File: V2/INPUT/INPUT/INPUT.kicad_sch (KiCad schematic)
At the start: 45 parts, among them J1 Conn_01x03, J2 USB_C_Receptacle_USB2.0_16P, J3 Conn_01x03, J4 Conn_01x03, J5 Conn_01x03, J6 Conn_01x03, J7 Conn_01x03, J8 Conn_01x03, J9 Conn_01x03, Q1 QM6006D, Q2 QM6006D, Q3 QM6006D, Q4 QM6006D, Q5 QM6006D, Q6 QM6006D, Q7 QM6006D, Q8 QM6006D, SW1 SW_SPST, SW2 SW_SPST, SW3 SW_SPST, SW4 SW_SPST, SW5 SW_SPST, SW6 SW_SPST, SW7 SW_SPST, SW8 SW_SPST, U1 USBLC6-2P6

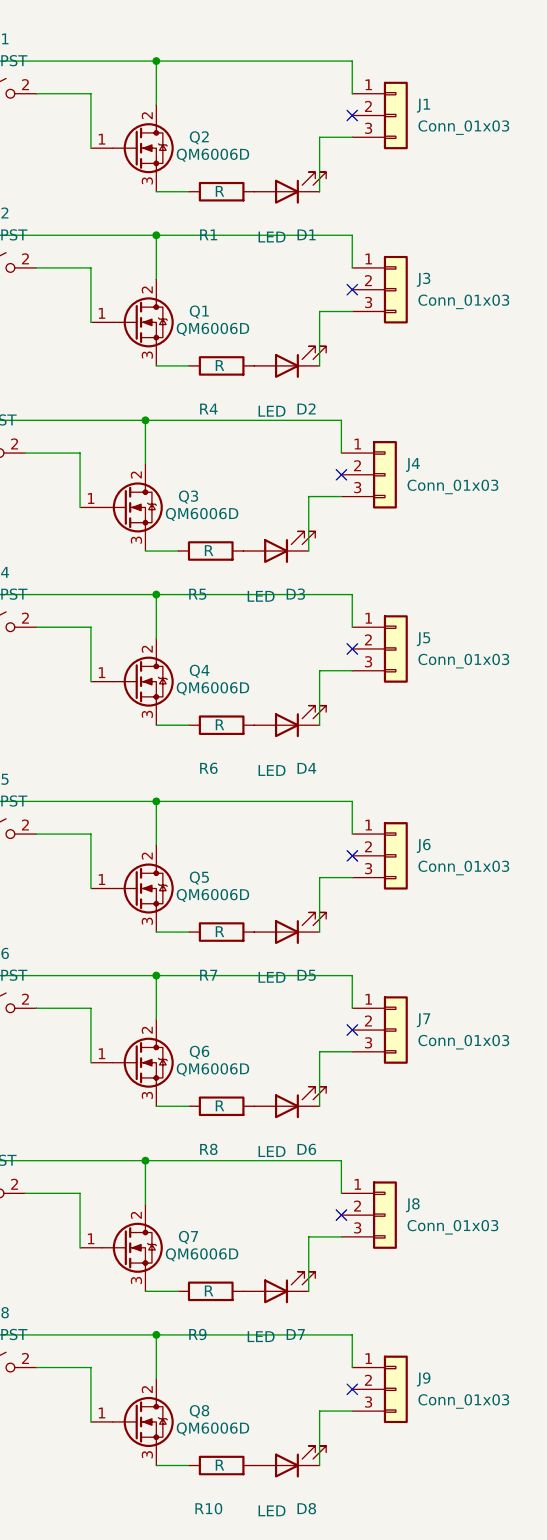
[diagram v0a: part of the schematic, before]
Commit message: Auto-update: 17.02.2026  0:08:41,99
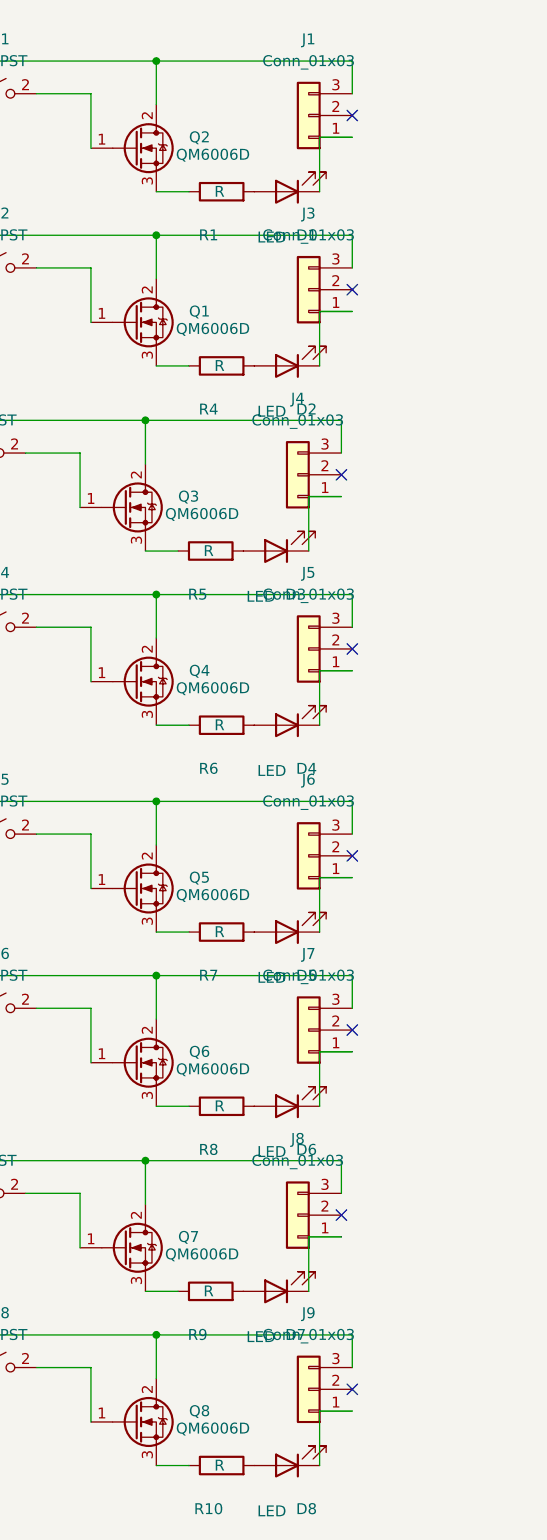
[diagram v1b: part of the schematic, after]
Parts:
- J1, J3, J4, J5, J6, J7, J8, J9: footprint Connector_JST:JST_PH_S3B-PH-K_1x03_P2.00mm_Horizontal -> Connector_PinSocket_2.54mm:PinSocket_1x03_P2.54mm_Horizontal
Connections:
- net +5V: now also J1.3 (Pin_3), J3.3 (Pin_3), J4.3 (Pin_3), J5.3 (Pin_3), J6.3 (Pin_3), J7.3 (Pin_3), J8.3 (Pin_3), J9.3 (Pin_3); no longer J1.1 (Pin_1), J3.1 (Pin_1), J4.1 (Pin_1), J5.1 (Pin_1), J6.1 (Pin_1), J7.1 (Pin_1), J8.1 (Pin_1), J9.1 (Pin_1)
- net at D6.1 (K): now also J7.1 (Pin_1); no longer J7.3 (Pin_3)
- net at D4.1 (K): now also J5.1 (Pin_1); no longer J5.3 (Pin_3)
- net at D1.1 (K): now also J1.1 (Pin_1); no longer J1.3 (Pin_3)
- net at D3.1 (K): now also J4.1 (Pin_1); no longer J4.3 (Pin_3)
- net at D2.1 (K): now also J3.1 (Pin_1); no longer J3.3 (Pin_3)
- net at D8.1 (K): now also J9.1 (Pin_1); no longer J9.3 (Pin_3)
- net at D5.1 (K): now also J6.1 (Pin_1); no longer J6.3 (Pin_3)
- net at D7.1 (K): now also J8.1 (Pin_1); no longer J8.3 (Pin_3)
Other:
- moved on the sheet: J1, J3, J4, J5, J6, J7, J8, J9

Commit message: Auto-update: 24.02.2026 16:00:58,58
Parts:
- Q1, Q2, Q3, Q4, Q5, Q6, Q7, Q8: footprint Package_TO_SOT_SMD:TO-252-2 -> Package_TO_SOT_SMD:SOT-23
- R1, R10, R2, R3, R4, R5, R6, R7, R8, R9: footprint Resistor_SMD:R_1206_3216Metric -> Resistor_SMD:R_0201_0603Metric
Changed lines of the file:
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@@
 			)
 		)
-		(property "Footprint" "Resistor_SMD:R_1206_3216Metric"
+		(property "Footprint" "Resistor_SMD:R_0201_0603Metric"
 			(at 132.08 185.928 90)
 			(effects
@@
 			)
 		)
-		(property "Footprint" "Resistor_SMD:R_1206_3216Metric"
+		(property "Footprint" "Resistor_SMD:R_0201_0603Metric"
 			(at 48.26 29.21 0)
 			(effects
@@
 			)
 		)
-		(property "Footprint" "Package_TO_SOT_SMD:TO-252-2"
+		(property "Footprint" "Package_TO_SOT_SMD:SOT-23"
 			(at 127 180.975 0)
 			(effects
@@
 			)
 		)
-		(property "Footprint" "Resistor_SMD:R_1206_3216Metric"
+		(property "Footprint" "Resistor_SMD:R_0201_0603Metric"
 			(at 132.08 144.018 90)
 			(effects
@@
 			)
 		)
-		(property "Footprint" "Resistor_SMD:R_1206_3216Metric"
+		(property "Footprint" "Resistor_SMD:R_0201_0603Metric"
 			(at 130.81 79.248 90)
 			(effects
@@
 			)
 		)
-		(property "Footprint" "Package_TO_SOT_SMD:TO-252-2"
+		(property "Footprint" "Package_TO_SOT_SMD:SOT-23"
 			(at 125.73 160.655 0)
 			(effects
@@
 			)
 		)
-		(property "Footprint" "Package_TO_SOT_SMD:TO-252-2"
+		(property "Footprint" "Package_TO_SOT_SMD:SOT-23"
 			(at 127 139.065 0)
 			(effects
@@
 			)
 		)
-		(property "Footprint" "Package_TO_SOT_SMD:TO-252-2"
+		(property "Footprint" "Package_TO_SOT_SMD:SOT-23"
 			(at 127 52.705 0)
 			(effects
@@
 			)
 		)
-		(property "Footprint" "Package_TO_SOT_SMD:TO-252-2"
+		(property "Footprint" "Package_TO_SOT_SMD:SOT-23"
 			(at 125.73 74.295 0)
 			(effects
@@
 			)
 		)
-		(property "Footprint" "Resistor_SMD:R_1206_3216Metric"
+		(property "Footprint" "Resistor_SMD:R_0201_0603Metric"
 			(at 130.81 165.608 90)
 			(effects
@@
 			)
 		)
-		(property "Footprint" "Resistor_SMD:R_1206_3216Metric"
+		(property "Footprint" "Resistor_SMD:R_0201_0603Metric"
 			(at 132.08 57.658 90)
 			(effects
@@
 			)
 		)
-		(property "Footprint" "Package_TO_SOT_SMD:TO-252-2"
+		(property "Footprint" "Package_TO_SOT_SMD:SOT-23"
 			(at 127 94.615 0)
 			(effects
@@
 			)
 		)
-		(property "Footprint" "Package_TO_SOT_SMD:TO-252-2"
+		(property "Footprint" "Package_TO_SOT_SMD:SOT-23"
 			(at 127 32.385 0)
 			(effects
@@
 			)
 		)
-		(property "Footprint" "Resistor_SMD:R_1206_3216Metric"
+		(property "Footprint" "Resistor_SMD:R_0201_0603Metric"
 			(at 132.08 123.698 90)
 			(effects
@@
 			)
 		)
-		(property "Footprint" "Resistor_SMD:R_1206_3216Metric"
+		(property "Footprint" "Resistor_SMD:R_0201_0603Metric"
 			(at 132.08 37.338 90)
 			(effects
@@
 			)
 		)
-		(property "Footprint" "Resistor_SMD:R_1206_3216Metric"
+		(property "Footprint" "Resistor_SMD:R_0201_0603Metric"
 			(at 132.08 99.568 90)
 			(effects
@@
 			)
 		)
-		(property "Footprint" "Package_TO_SOT_SMD:TO-252-2"
+		(property "Footprint" "Package_TO_SOT_SMD:SOT-23"
 			(at 127 118.745 0)
 			(effects
@@
 			)
 		)
-		(property "Footprint" "Resistor_SMD:R_1206_3216Metric"
+		(property "Footprint" "Resistor_SMD:R_0201_0603Metric"
 			(at 48.26 31.75 0)
 			(effects

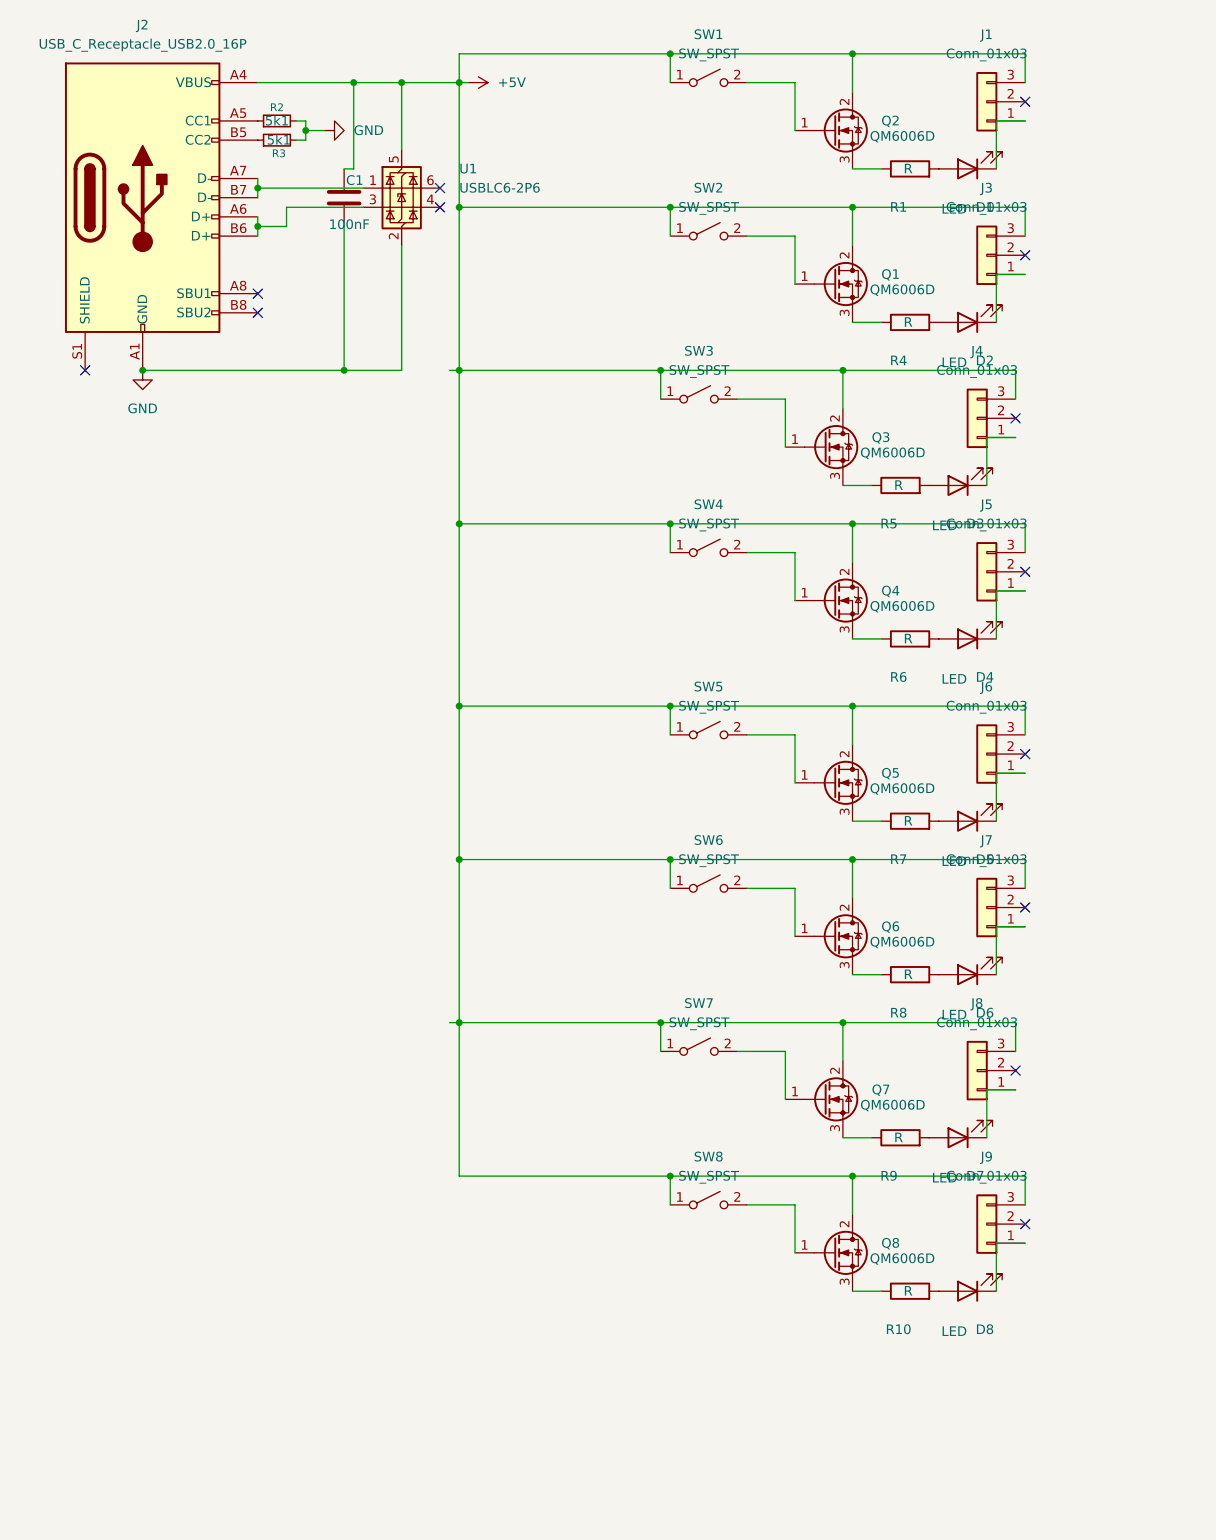
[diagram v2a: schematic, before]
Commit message: Auto-update: 26.02.2026  0:22:57,46
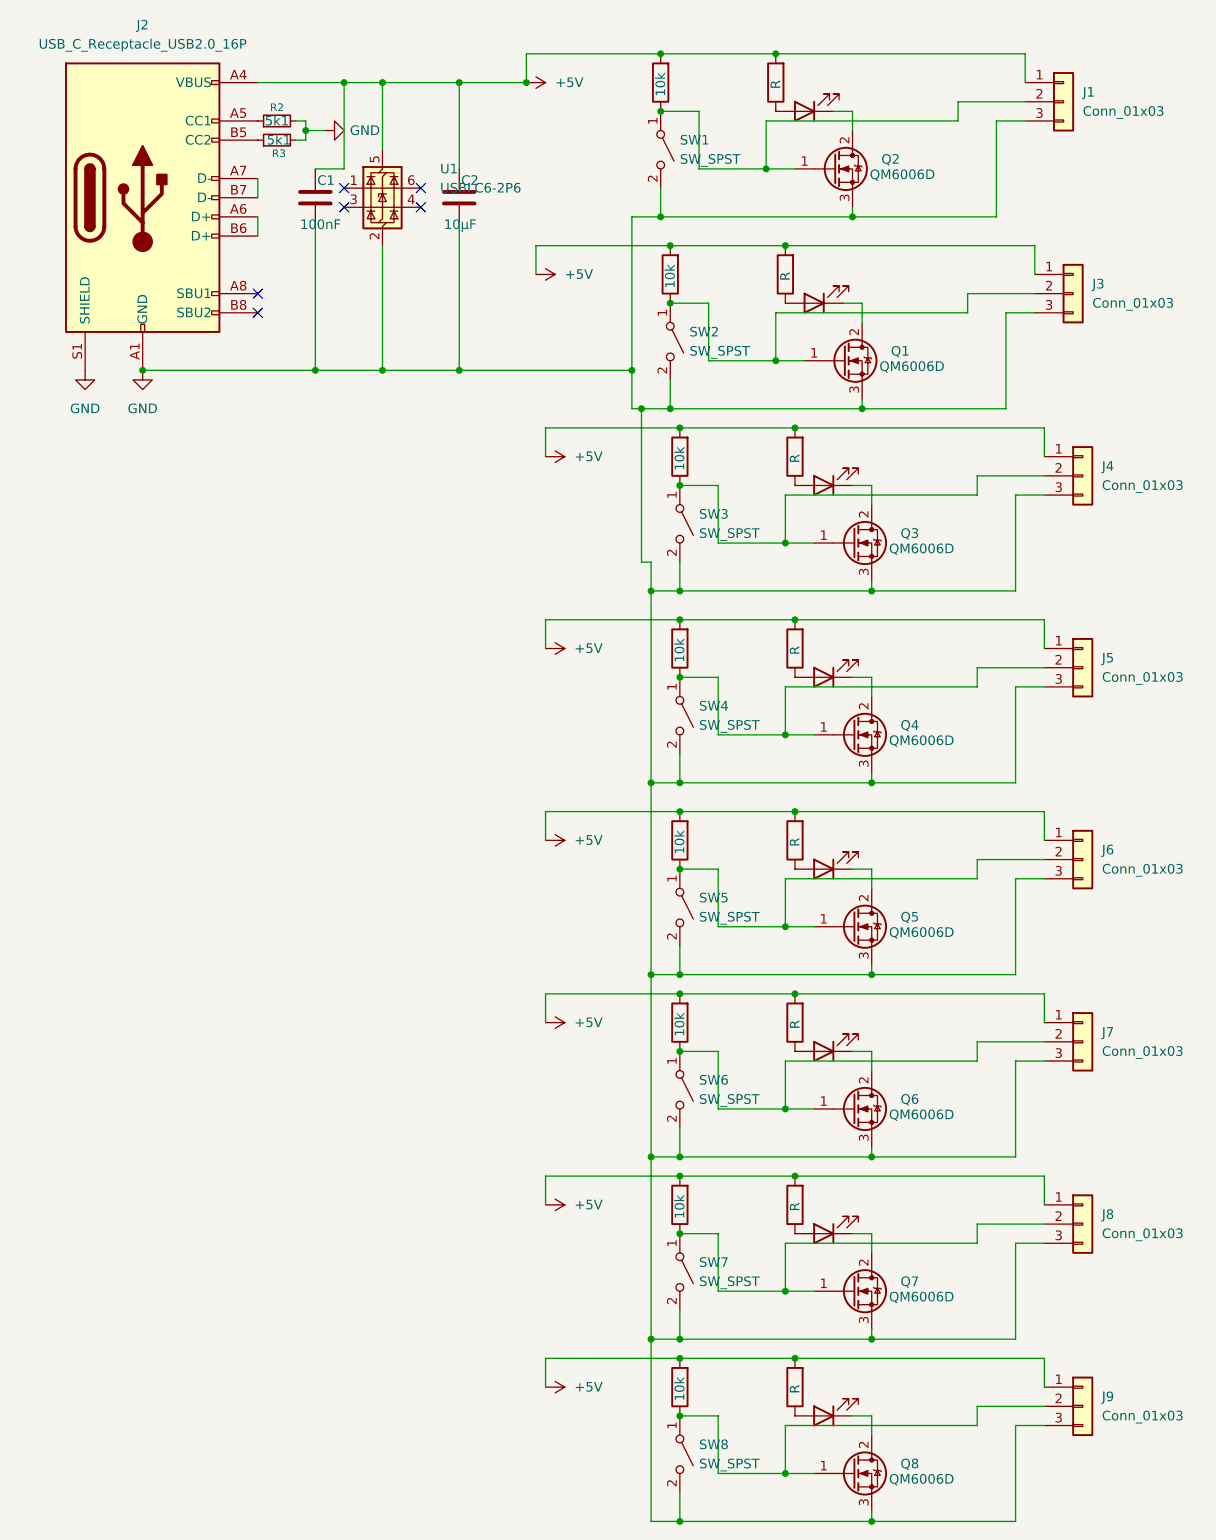
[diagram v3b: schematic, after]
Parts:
- added C2: 10µF, Capacitor_SMD:C_1206_3216Metric, symbol Device:C
- added R11, R13, R15, R17: 10k, Resistor_SMD:R_0201_0603Metric, symbol Device:R
- added R12, R14, R16, R18: R, Resistor_SMD:R_0201_0603Metric, symbol Device:R
- C1: footprint Capacitor_SMD:C_1206_3216Metric -> Capacitor_SMD:C_0201_0603Metric
- R4, R5, R7, R9: value R -> 10k
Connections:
- net +5V: now also J1.1 (Pin_1), J3.1 (Pin_1), J4.1 (Pin_1), J5.1 (Pin_1), J6.1 (Pin_1), J7.1 (Pin_1), J8.1 (Pin_1), J9.1 (Pin_1), R1.2, R10.2, R4.2, R5.2, R6.2, R7.2, R8.2, R9.2, C2.1, R11.2, R12.2, R13.2, R14.2, R15.2, R16.2, R17.2, R18.2; no longer J1.3 (Pin_3), J3.3 (Pin_3), J4.3 (Pin_3), J5.3 (Pin_3), J6.3 (Pin_3), J7.3 (Pin_3), J8.3 (Pin_3), J9.3 (Pin_3), Q1.2 (D), Q2.2 (D), Q3.2 (D), Q4.2 (D), Q5.2 (D), Q6.2 (D), Q7.2 (D), Q8.2 (D), SW1.1 (A), SW2.1 (A), SW3.1 (A), SW4.1 (A), SW5.1 (A), SW6.1 (A), SW7.1 (A), SW8.1 (A)
- net GND: now also J1.3 (Pin_3), J2.S1 (SHIELD), J3.3 (Pin_3), J4.3 (Pin_3), J5.3 (Pin_3), J6.3 (Pin_3), J7.3 (Pin_3), J8.3 (Pin_3), J9.3 (Pin_3), Q1.3 (S), Q2.3 (S), Q3.3 (S), Q4.3 (S), Q5.3 (S), Q6.3 (S), Q7.3 (S), Q8.3 (S), SW1.2 (B), SW2.2 (B), SW3.2 (B), SW4.2 (B), SW5.2 (B), SW6.2 (B), SW7.2 (B), SW8.2 (B), C2.2
- net at R10.1: now also D4.2 (A); no longer Q8.3 (S)
- net at D8.2 (A): now also R18.1; no longer R10.2
- net at Q8.1 (G): now also J9.2 (Pin_2), SW8.1 (A), R17.1; no longer SW8.2 (B)
- net at Q7.1 (G): now also J8.2 (Pin_2), SW7.1 (A), R15.1; no longer SW7.2 (B)
- net at R8.1: now also D3.2 (A); no longer Q6.3 (S)
- net at D6.2 (A): now also R14.1; no longer R8.2
- net at D6.1 (K): now also Q6.2 (D); no longer J7.1 (Pin_1)
- net at D4.1 (K): now also Q4.2 (D); no longer J5.1 (Pin_1)
- net at D1.1 (K): now also Q2.2 (D); no longer J1.1 (Pin_1)
- net at D1.2 (A): now also R1.1; no longer R1.2
- net at D3.1 (K): now also Q3.2 (D); no longer J4.1 (Pin_1)
- net at R5.1: now also J3.2 (Pin_2), Q1.1 (G), SW2.1 (A); no longer Q3.3 (S)
- net at R9.1: now also J5.2 (Pin_2), Q4.1 (G), SW4.1 (A); no longer Q7.3 (S)
- net at D2.1 (K): now also Q1.2 (D); no longer J3.1 (Pin_1)
- net at D8.1 (K): now also Q8.2 (D); no longer J9.1 (Pin_1)
- net at Q6.1 (G): now also J7.2 (Pin_2), SW6.1 (A), R13.1; no longer SW6.2 (B)
- net at J1.2 (Pin_2): now also Q2.1 (G), R4.1, SW1.1 (A)
- net at D5.1 (K): now also Q5.2 (D); no longer J6.1 (Pin_1)
- net at D5.2 (A): now also R12.1; no longer R7.2
- net at J2.A7 (D-), J2.B7 (D-): no longer U1.1 (I/O1)
- net at J2.A6 (D+), J2.B6 (D+): no longer U1.3 (I/O2)
- net at Q3.1 (G): now also J4.2 (Pin_2), R7.1, SW3.1 (A); no longer SW3.2 (B)
- net at D7.2 (A): now also R16.1; no longer R9.2
- net at D2.2 (A): now also R6.1; no longer R4.2
- net at D7.1 (K): now also Q7.2 (D); no longer J8.1 (Pin_1)
- net at Q5.1 (G): now also J6.2 (Pin_2), SW5.1 (A), R11.1; no longer SW5.2 (B)
- no-connect marks 13 -> 6
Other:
- moved on the sheet: C1, J1, Q2, SW1, U1
